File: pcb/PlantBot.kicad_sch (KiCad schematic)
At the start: 0 parts

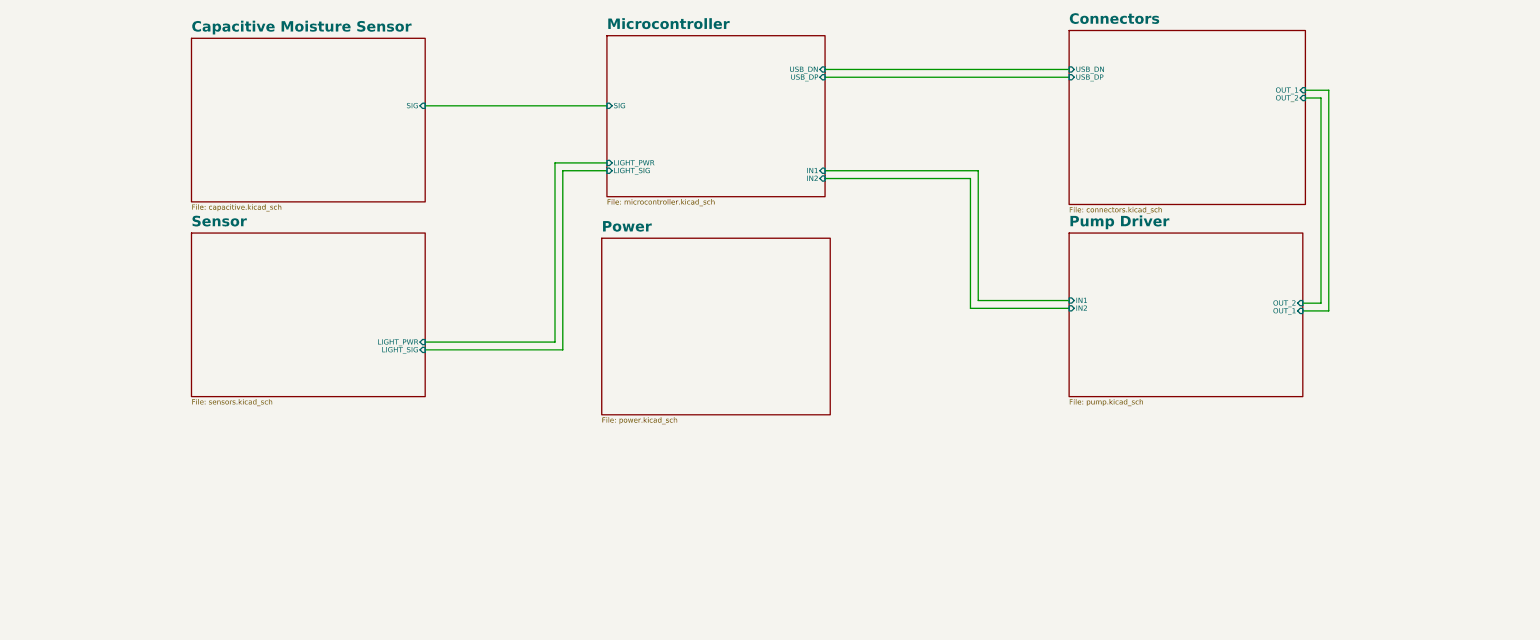
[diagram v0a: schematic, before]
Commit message: Completed initial schematic
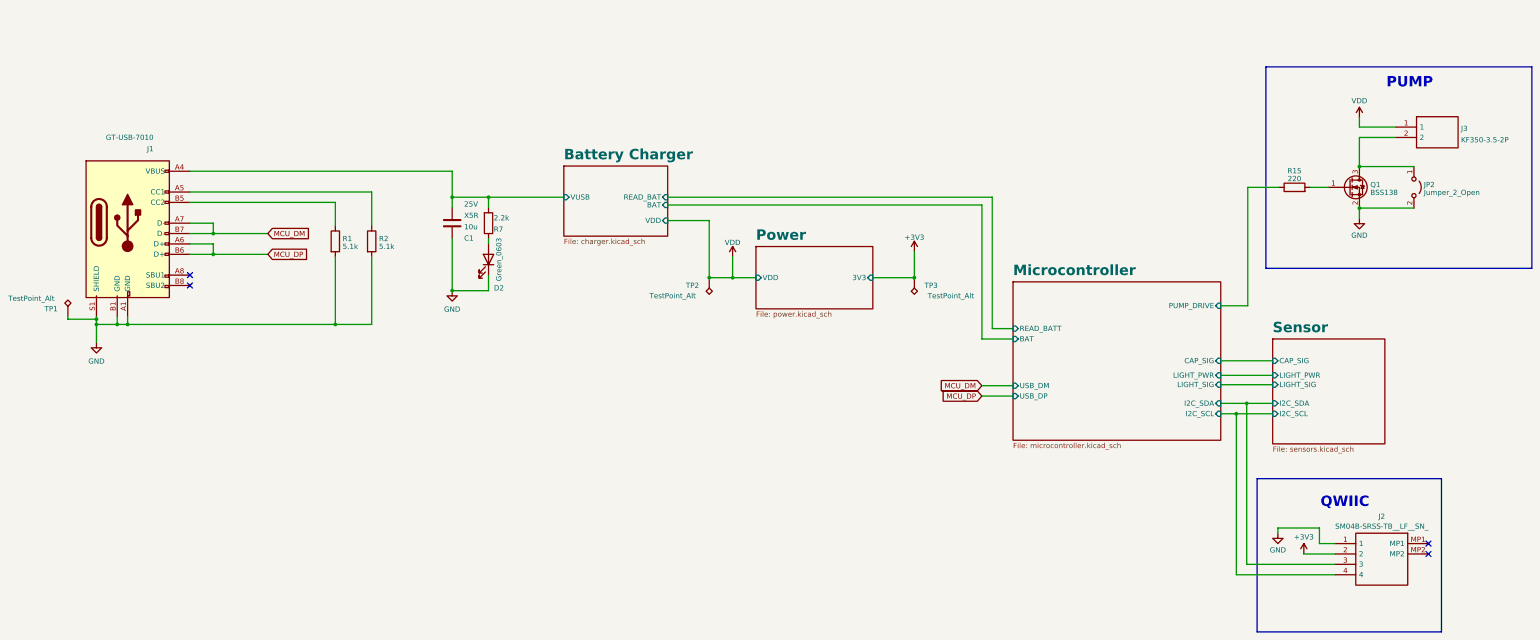
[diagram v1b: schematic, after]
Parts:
- added C1: 10u, Capacitor_SMD:C_0805_2012Metric, symbol Capacitor_JLC:10u
- added D2: Green_0603, LED_SMD:LED_0603_1608Metric, symbol Diode_JLC:Green_0603
- added J1: GT-USB-7010, Connectors_JT:GT-USB-7010A, symbol Connector_JLC:GT-USB-7010
- added J2: SM04B-SRSS-TB__LF__SN_, SM04BSRSSTBLFSN, symbol Connector_JLC:SM04B-SRSS-TB__LF__SN_
- added J3: KF350-3.5-2P, KF350352P, symbol Connector_JLC:KF350-3.5-2P
- added JP2: Jumper_2_Open, Jumper:SolderJumper-2_P1.3mm_Open_RoundedPad1.0x1.5mm, symbol Jumper:Jumper_2_Open
- added Q1: BSS138, Package_TO_SOT_SMD:SOT-23, symbol Transistor_JLC:BSS138
- added R1, R2: 5.1k, Resistor_SMD:R_0402_1005Metric, symbol Resistor_JLC:5.1k
- added R15: 220, Resistor_SMD:R_0402_1005Metric, symbol Resistor_JLC:220
- added R7: 2.2k, Resistor_SMD:R_0402_1005Metric, symbol Resistor_JLC:2.2k
- added TP1, TP2, TP3: TestPoint_Alt, TestPoint:TestPoint_Pad_1.0x1.0mm, symbol personal:TestPoint_Alt
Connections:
- new net: D2.2 (A), R7.1
- new net: J1.A5 (CC1), R2.1
- new net: J3.2, JP2.1 (A), Q1.3 (D)
- new net: J1.B5 (CC2), R1.1
- new net: Q1.1 (G), R15.2
- new net +3V3: J2.2, TP3.1
- new net Battery Charger/VUSB: C1.2, J1.A4 (VBUS), J1.A9 (VBUS), J1.B4 (VBUS), J1.B9 (VBUS), R7.2
- new net GND: C1.1, D2.1 (K), J1.A1 (GND), J1.B1 (GND), J1.S1 (SHIELD), J2.1, JP2.2 (B), Q1.2 (S), R1.2, R2.2, TP1.1
- new net MCU_DM: J1.A7 (D-), J1.B7 (D-)
- new net MCU_DP: J1.A6 (D+), J1.B6 (D+)
- new net Microcontroller/I2C_SCL: J2.4
- new net Microcontroller/I2C_SDA: J2.3
- new net Microcontroller/PUMP_DRIVE: R15.1
- new net VDD: J3.1, TP2.1
- no-connect marks 0 -> 4
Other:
- removed sheet Capacitive Moisture Sensor
- removed sheet Connectors
- removed sheet Pump Driver
- added sheet Battery Charger (charger.kicad_sch)
- sheet Microcontroller ports: added BAT, CAP_SIG, I2C_SCL, I2C_SDA, PUMP_DRIVE, READ_BATT, USB_DM; removed IN1, IN2, SIG, USB_DN
- sheet Power ports: added 3V3, VDD; removed none
- sheet Sensor ports: added CAP_SIG, I2C_SCL, I2C_SDA; removed none
- note added: "PUMP"
- note added: "QWIIC"
